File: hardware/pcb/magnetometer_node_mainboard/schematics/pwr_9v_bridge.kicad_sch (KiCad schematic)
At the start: 0 parts

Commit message: Schematic sensor stage done
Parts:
- added U5: LT3042xMSE, Package_SO:MSOP-10-1EP_3x3mm_P0.5mm_EP1.68x1.88mm, symbol Regulator_Linear:LT3042xMSE
- added U6: TPS61040DBV, Package_TO_SOT_SMD:SOT-23-5, symbol Regulator_Switching:TPS61040DBV
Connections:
- new net: U5.1 (IN), U5.2 (IN)
- new net: U5.11 (GND), U5.8 (GND)
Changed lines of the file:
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@@
 	(generator_version "9.0")
 	(paper "A4")
+	(symbol
+		(lib_id "Regulator_Linear:LT3042xMSE")
+		(at 132.08 80.01 0)
+		(unit 1)
+		(exclude_from_sim no)
+		(in_bom yes)
+		(on_board yes)
+		(dnp no)
+		(fields_autoplaced yes)
+		(property "Reference" "U5"
+			(at 132.08 69.85 0)
+			(effects
+				(font
+					(size 1.27 1.27)
+				)
+			)
+		)
+		(property "Value" "LT3042xMSE"
+			(at 132.08 72.39 0)
+			(effects
+				(font
+					(size 1.27 1.27)
+				)
+			)
+		)
+		(property "Footprint" "Package_SO:MSOP-10-1EP_3x3mm_P0.5mm_EP1.68x1.88mm"
+			(at 132.08 71.755 0)
+			(effects
+				(font
+					(size 1.27 1.27)
+				)
+				(hide yes)
+			)
+		)
+		(property "Datasheet" "https://www.analog.com/media/en/technical-documentation/data-sheets/3042fb.pdf"
+			(at 132.08 80.01 0)
+			(effects
+				(font
+					(size 1.27 1.27)
+				)
+				(hide yes)
+			)
+		)
+		(property "Description" "200mA, Adjustable, Ultralow Noise, Ultrahigh PSRR RF Linear Regulator, MSOP-10"
+			(at 132.08 80.01 0)
+			(effects
+				(font
+					(size 1.27 1.27)
+				)
+				(hide yes)
+			)
+		)
+		(pin "5"
+		)
+		(pin "3"
+		)
+		(pin "8"
+		)
+		(pin "10"
+		)
+		(pin "9"
+		)
+		(pin "6"
+		)
+		(pin "1"
+		)
+		(pin "2"
+		)
+		(pin "11"
+		)
+		(pin "4"
+		)
+		(pin "7"
+		)
+		(instances
+			(project ""
+				(path "/b5f9ef85-43f0-43d8-a1fd-ed489b1654c1/ded83d55-b2f7-490a-b9dc-0b3a44a3cee5"
+					(reference "U5")
+					(unit 1)
+				)
+			)
+		)
+	)
+	(symbol
+		(lib_id "Regulator_Switching:TPS61040DBV")
+		(at 88.9 80.01 0)
+		(unit 1)
+		(exclude_from_sim no)
+		(in_bom yes)
+		(on_board yes)
+		(dnp no)
+		(fields_autoplaced yes)
+		(property "Reference" "U6"
+			(at 88.9 69.85 0)
+			(effects
+				(font
+					(size 1.27 1.27)
+				)
+			)
+		)
+		(property "Value" "TPS61040DBV"
+			(at 88.9 72.39 0)
+			(effects
+				(font
+					(size 1.27 1.27)
+				)
+			)
+		)
+		(property "Footprint" "Package_TO_SOT_SMD:SOT-23-5"
+			(at 91.44 86.36 0)
+			(effects
+				(font
+					(size 1.27 1.27)
+					(italic yes)
+				)
+				(justify left)
+				(hide yes)
+			)
+		)
+		(property "Datasheet" "http://www.ti.com/lit/ds/symlink/tps61040.pdf"
+			(at 83.82 72.39 0)
+			(effects
+				(font
+					(size 1.27 1.27)
+				)
+				(hide yes)
+			)
+		)
+		(property "Description" "Synchronous Boost Regulator, Adjustable Output up to 28V, 400 mA Switch Current Limit, SOT-23-5"
+			(at 88.9 80.01 0)
+			(effects
+				(font
+					(size 1.27 1.27)
+				)
+				(hide yes)
+			)
+		)
+		(pin "4"
+		)
+		(pin "5"
+		)
+		(pin "3"
+		)
+		(pin "2"
+		)
+		(pin "1"
+		)
+		(instances
+			(project ""
+				(path "/b5f9ef85-43f0-43d8-a1fd-ed489b1654c1/ded83d55-b2f7-490a-b9dc-0b3a44a3cee5"
+					(reference "U6")
+					(unit 1)
+				)
+			)
+		)
+	)
 )

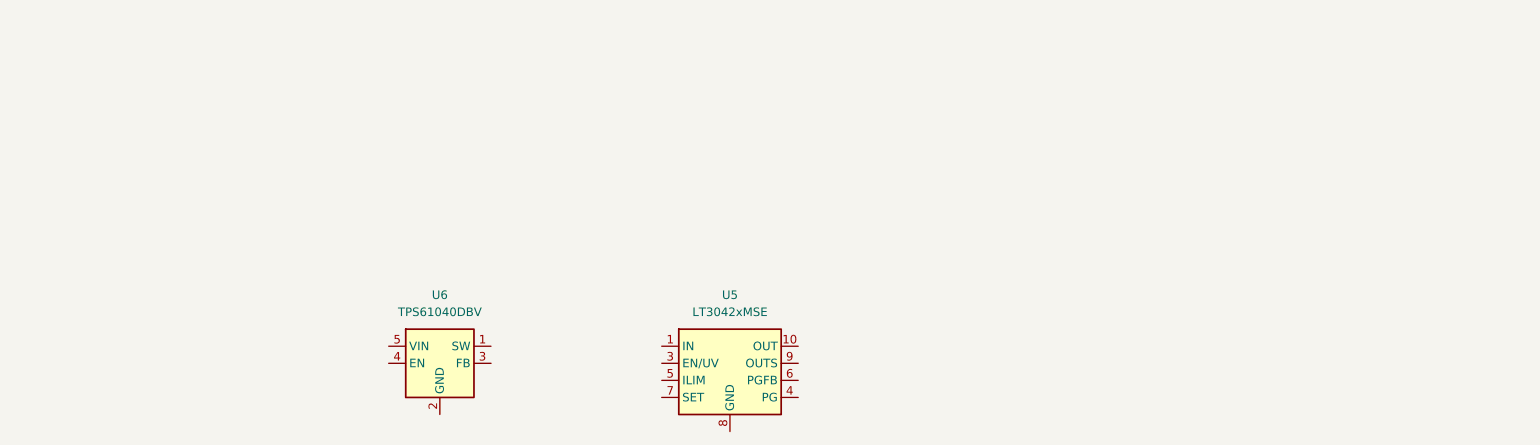
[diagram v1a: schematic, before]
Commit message: first code for the v1
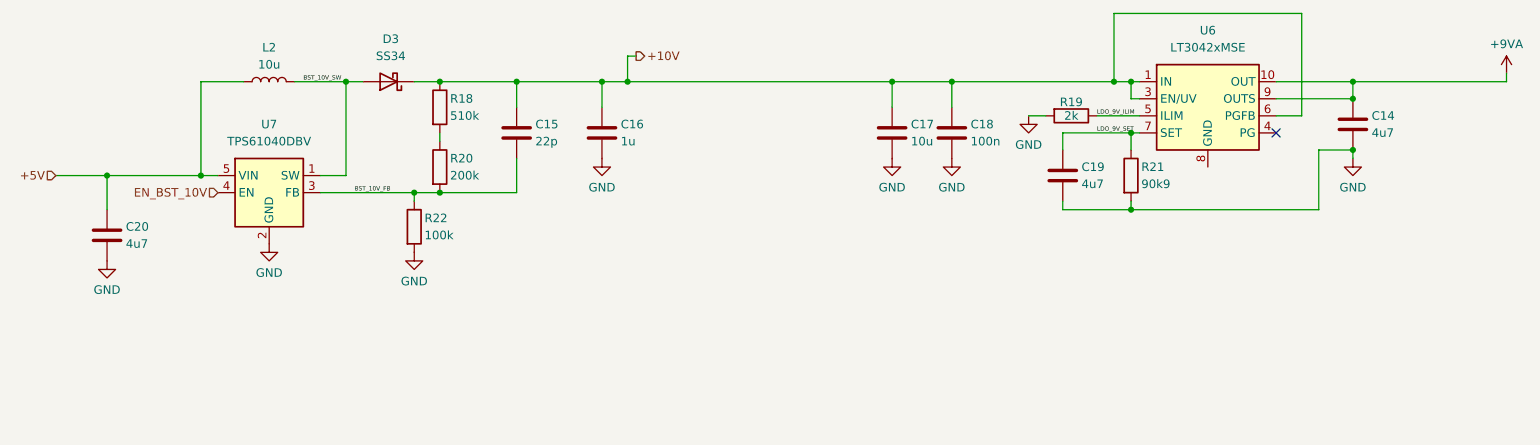
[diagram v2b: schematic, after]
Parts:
- added C14, C19, C20: 4u7, Capacitor_SMD:C_1206_3216Metric, symbol Device:C
- added C15: 22p, Capacitor_SMD:C_0603_1608Metric, symbol Device:C
- added C16: 1u, Capacitor_SMD:C_0805_2012Metric, symbol Device:C
- added C17: 10u, Capacitor_SMD:C_0805_2012Metric, symbol Device:C
- added C18: 100n, Capacitor_SMD:C_0603_1608Metric, symbol Device:C
- added D3: SS34, Diode_SMD:D_SMA, symbol Device:D_Schottky
- added L2: 10u, Capacitor_SMD:C_0805_2012Metric, symbol Device:L
- added R18: 510k, Resistor_SMD:R_0603_1608Metric, symbol Device:R
- added R19: 2k, Resistor_SMD:R_0603_1608Metric, symbol Device:R
- added R20: 200k, Resistor_SMD:R_0603_1608Metric, symbol Device:R
- added R21: 90k9, Resistor_SMD:R_1206_3216Metric, symbol Device:R
- added R22: 100k, Resistor_SMD:R_0603_1608Metric, symbol Device:R
- renumbered U5 to U6, U6 to U7
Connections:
- net +10V: now reaches U6.1 (IN), U6.2 (IN)
- net +10V: now also U6.3 (EN/UV), U6.6 (PGFB), C15.1, C16.1, C17.1, C18.1, D3.1 (K), R18.1
- net +9VA: now reaches U6.10 (OUT)
- net +9VA: now also U6.9 (OUTS), C14.1
- net LDO_9V_ILIM: now reaches U6.5 (ILIM)
- net LDO_9V_ILIM: now also R19.1
- net LDO_9V_SET: now reaches U6.7 (SET)
- net LDO_9V_SET: now also C19.1, R21.1
- net BST_10V_SW: now reaches U7.1 (SW)
- net BST_10V_SW: now also D3.2 (A), L2.2
- net GND: now reaches U7.2 (GND)
- net GND: now also C14.2, C16.2, C17.2, C18.2, C19.2, C20.2, R19.2, R21.2, R22.2
- net BST_10V_FB: now reaches U7.3 (FB)
- net BST_10V_FB: now also C15.2, R20.2, R22.1
- net EN_BST_10V: now reaches U7.4 (EN)
- net +5V: now reaches U7.5 (VIN)
- net +5V: now also C20.1, L2.1
- new net: R18.2, R20.1
- no-connect marks 0 -> 1
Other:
- moved on the sheet: U6, U7
